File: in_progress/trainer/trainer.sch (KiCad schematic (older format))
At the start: 58 parts, among them CON1 BARREL_JACK, P1 CONN_01X04, P2 CONN_01X02, P3 CONN_01X03, P4 USB_A, P5 CONN_01X02, P6 CONN_01X03, P7 CONN_02X08, Q1 2N3904, U1 ULN2803A, U2 LM7805, U3 ULN2803A, U4 ULN2803A, X1 Buzzer_Son

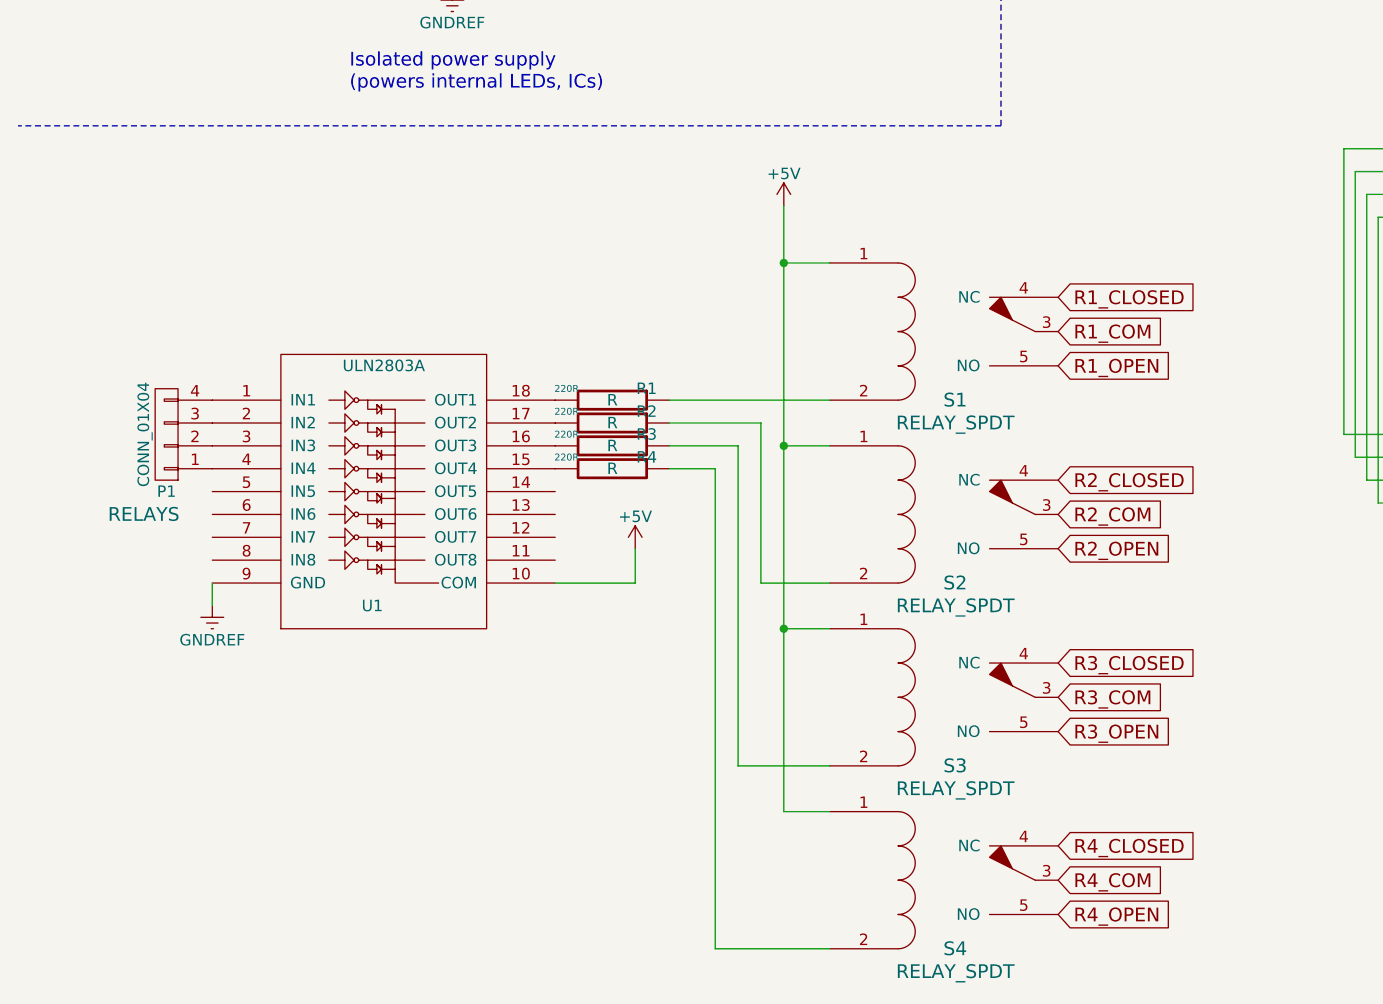
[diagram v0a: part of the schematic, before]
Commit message: .
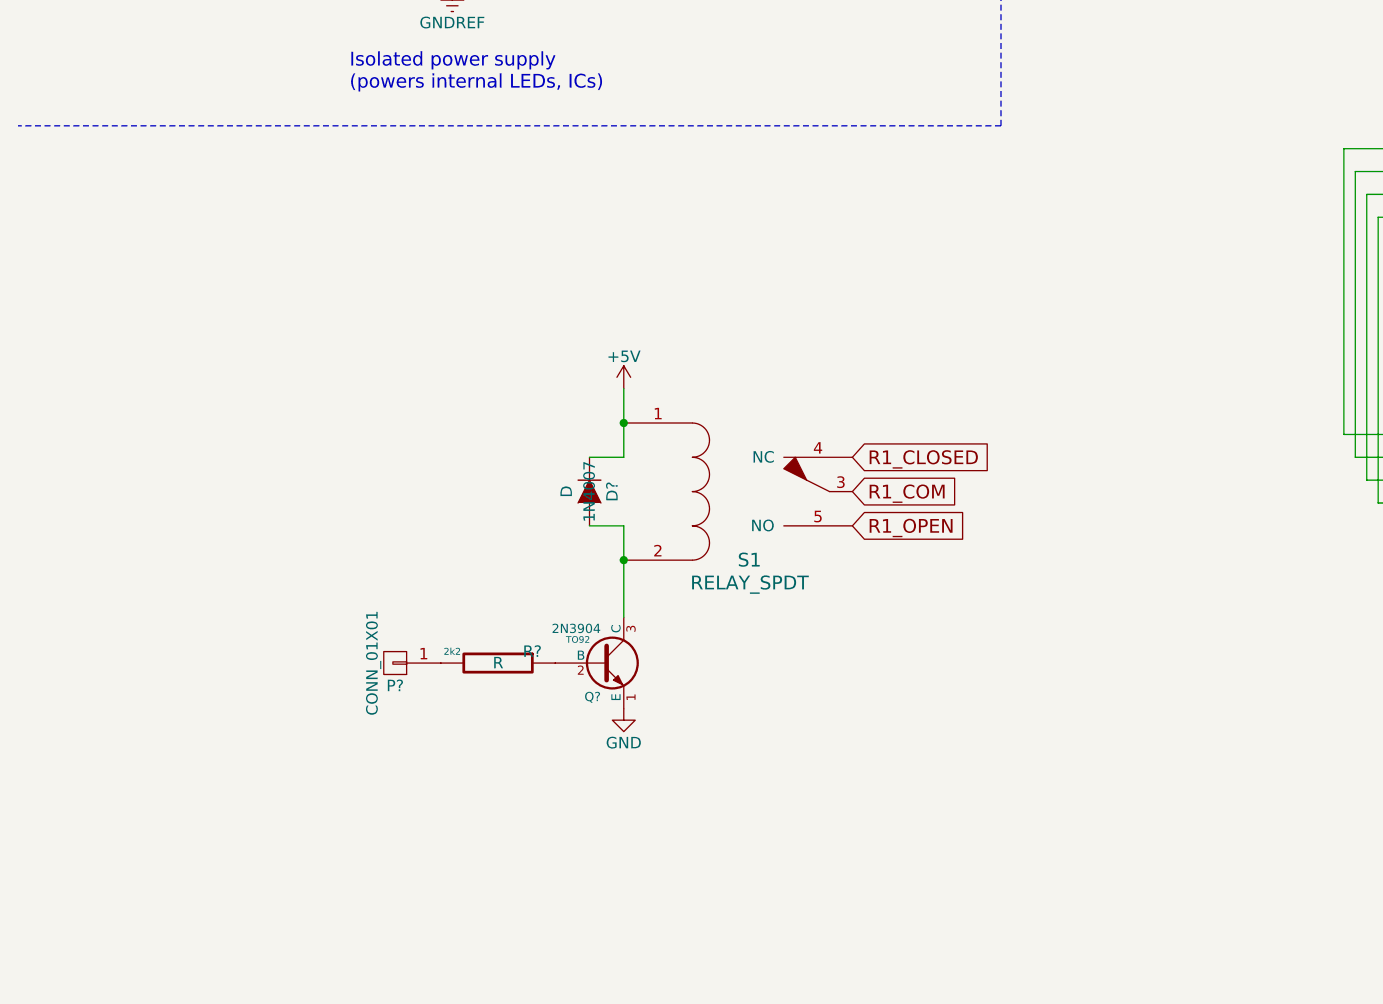
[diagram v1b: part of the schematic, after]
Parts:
- removed P1: CONN_01X04, RELAYS, symbol CONN_01X04
- removed R1, R2, R3, R4: R, 220R, symbol R-RESCUE-trainer
- removed S2, S3, S4: RELAY_SPDT, symbol RELAY_SPDT
- removed U1: ULN2803A, symbol ULN2803A
- added D?: D, 1N4007, symbol D
- added P?: CONN_01X01, symbol CONN_01X01
- added Q?: 2N3904, TO92, symbol PN2222A-RESCUE-trainer
- added R?: R, 2k2, symbol R-RESCUE-trainer
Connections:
- net labels removed: R2_CLOSED, R2_COM, R2_OPEN, R3_CLOSED, R3_COM, R3_OPEN, R4_CLOSED, R4_COM, R4_OPEN
- wire segments 123 -> 109
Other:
- moved on the sheet: S1
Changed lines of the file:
@@
 F1 "inputs.sch" 60
 $EndSheet
-$Comp
-L RELAY_SPDT S1
-U 1 1 56568F0F
-P 4700 4450
-F 0 "S1" H 4700 4150 60  0000 C CNN
-F 1 "RELAY_SPDT" H 4700 4050 60  0000 C CNN
-F 2 "" H 4700 4450 60  0000 C CNN
-F 3 "" H 4700 4450 60  0000 C CNN
-	1    4700 4450
-	1    0    0    -1
-$EndComp
-$Comp
-L CONN_01X04 P1
-U 1 1 5656959C
-P 1250 4900
-F 0 "P1" H 1250 5150 50  0000 C CNN
-F 1 "CONN_01X04" V 1350 4900 50  0000 C CNN
-F 2 "RELAYS" H 1350 5250 60  0000 C CNN
-F 3 "" H 1250 4900 60  0000 C CNN
-	1    1250 4900
-	-1   0    0    1
-$EndComp
-Text GLabel 5150 4300 2    60   Input ~ 0
+Text GLabel 4250 5000 2    60   Input ~ 0
 R1_CLOSED
-Text GLabel 5150 4450 2    60   Input ~ 0
+Text GLabel 4250 5150 2    60   Input ~ 0
 R1_COM
-Text GLabel 5150 4600 2    60   Input ~ 0
+Text GLabel 4250 5300 2    60   Input ~ 0
 R1_OPEN
-$Comp
-L RELAY_SPDT S2
-U 1 1 5656BF1B
-P 4700 5250
-F 0 "S2" H 4700 4950 60  0000 C CNN
-F 1 "RELAY_SPDT" H 4700 4850 60  0000 C CNN
-F 2 "" H 4700 5250 60  0000 C CNN
-F 3 "" H 4700 5250 60  0000 C CNN
-	1    4700 5250
-	1    0    0    -1
-$EndComp
-Text GLabel 5150 5100 2    60   Input ~ 0
-R2_CLOSED
-Text GLabel 5150 5250 2    60   Input ~ 0
-R2_COM
-Text GLabel 5150 5400 2    60   Input ~ 0
-R2_OPEN
-$Comp
-L RELAY_SPDT S3
-U 1 1 5656C278
-P 4700 6050
-F 0 "S3" H 4700 5750 60  0000 C CNN
-F 1 "RELAY_SPDT" H 4700 5650 60  0000 C CNN
-F 2 "" H 4700 6050 60  0000 C CNN
-F 3 "" H 4700 6050 60  0000 C CNN
-	1    4700 6050
-	1    0    0    -1
-$EndComp
-Text GLabel 5150 5900 2    60   Input ~ 0
-R3_CLOSED
-Text GLabel 5150 6050 2    60   Input ~ 0
-R3_COM
-Text GLabel 5150 6200 2    60   Input ~ 0
-R3_OPEN
-$Comp
-L RELAY_SPDT S4
-U 1 1 5656C28D
-P 4700 6850
-F 0 "S4" H 4700 6550 60  0000 C CNN
-F 1 "RELAY_SPDT" H 4700 6450 60  0000 C CNN
-F 2 "" H 4700 6850 60  0000 C CNN
-F 3 "" H 4700 6850 60  0000 C CNN
-	1    4700 6850
-	1    0    0    -1
-$EndComp
-Text GLabel 5150 6700 2    60   Input ~ 0
-R4_CLOSED
-Text GLabel 5150 6850 2    60   Input ~ 0
-R4_COM
-Text GLabel 5150 7000 2    60   Input ~ 0
-R4_OPEN
 $Comp
 L LM7805 U2
@@
 $EndComp
 $Comp
-L R-RESCUE-trainer R1
-U 1 1 5659DCCE
-P 3200 4750
-F 0 "R1" V 3150 4900 50  0000 C CNN
-F 1 "R" V 3200 4750 50  0000 C CNN
-F 2 "220R" V 3150 4550 30  0000 C CNN
-F 3 "" H 3200 4750 30  0000 C CNN
-	1    3200 4750
-	0    1    1    0
-$EndComp
-$Comp
-L R-RESCUE-trainer R2
-U 1 1 5659E1A6
-P 3200 4850
-F 0 "R2" V 3150 5000 50  0000 C CNN
-F 1 "R" V 3200 4850 50  0000 C CNN
-F 2 "220R" V 3150 4650 30  0000 C CNN
-F 3 "" H 3200 4850 30  0000 C CNN
-	1    3200 4850
-	0    1    1    0
-$EndComp
-$Comp
-L R-RESCUE-trainer R3
-U 1 1 5659E1E3
-P 3200 4950
-F 0 "R3" V 3150 5100 50  0000 C CNN
-F 1 "R" V 3200 4950 50  0000 C CNN
-F 2 "220R" V 3150 4750 30  0000 C CNN
-F 3 "" H 3200 4950 30  0000 C CNN
-	1    3200 4950
-	0    1    1    0
-$EndComp
-$Comp
-L R-RESCUE-trainer R4
-U 1 1 5659E227
-P 3200 5050
-F 0 "R4" V 3150 5200 50  0000 C CNN
-F 1 "R" V 3200 5050 50  0000 C CNN
-F 2 "220R" V 3150 4850 30  0000 C CNN
-F 3 "" H 3200 5050 30  0000 C CNN
-	1    3200 5050
-	0    1    1    0
-$EndComp
-$Comp
-L ULN2803A U1
-U 1 1 5659B908
-P 2200 5150
-F 0 "U1" H 2150 4650 50  0000 C CNN
-F 1 "ULN2803A" H 2200 5700 50  0000 C CNN
-F 2 "" H 2200 5150 60  0000 C CNN
-F 3 "" H 2200 5150 60  0000 C CNN
-	1    2200 5150
-	1    0    0    -1
-$EndComp
-$Comp
 L +5V #PWR8
 U 1 1 565A0518
-P 3950 3900
-F 0 "#PWR8" H 3950 3750 50  0001 C CNN
-F 1 "+5V" H 3950 4040 50  0000 C CNN
-F 2 "" H 3950 3900 60  0000 C CNN
-F 3 "" H 3950 3900 60  0000 C CNN
-	1    3950 3900
-	1    0    0    -1
-$EndComp
-$Comp
-L GNDREF #PWR3
-U 1 1 565A1ACC
-P 1450 5650
-F 0 "#PWR3" H 1450 5400 50  0001 C CNN
-F 1 "GNDREF" H 1450 5500 50  0000 C CNN
-F 2 "" H 1450 5650 60  0000 C CNN
-F 3 "" H 1450 5650 60  0000 C CNN
-	1    1450 5650
-	1    0    0    -1
-$EndComp
-$Comp
-L +5V #PWR6
-U 1 1 565A1B8D
-P 3300 5400
-F 0 "#PWR6" H 3300 5250 50  0001 C CNN
-F 1 "+5V" H 3300 5540 50  0000 C CNN
-F 2 "" H 3300 5400 60  0000 C CNN
-F 3 "" H 3300 5400 60  0000 C CNN
-	1    3300 5400
+P 3250 4700
+F 0 "#PWR8" H 3250 4550 50  0001 C CNN
+F 1 "+5V" H 3250 4840 50  0000 C CNN
+F 2 "" H 3250 4700 60  0000 C CNN
+F 3 "" H 3250 4700 60  0000 C CNN
+	1    3250 4700
 	1    0    0    -1
 $EndComp
@@
 	3500 2850 3500 2500
 Wire Wire Line
-	3950 3900 3950 6550
-Wire Wire Line
-	3950 4150 4150 4150
-Wire Wire Line
-	3950 4950 4150 4950
-Connection ~ 3950 4150
-Wire Wire Line
-	3950 5750 4150 5750
-Connection ~ 3950 4950
-Wire Wire Line
-	3950 6550 4150 6550
-Connection ~ 3950 5750
-Wire Wire Line
-	4150 4750 3450 4750
-Wire Wire Line
-	4150 5550 3850 5550
-Wire Wire Line
-	3850 5550 3850 4850
-Wire Wire Line
-	3850 4850 3450 4850
-Wire Wire Line
-	4150 6350 3750 6350
-Wire Wire Line
-	3750 6350 3750 4950
-Wire Wire Line
-	3750 4950 3450 4950
-Wire Wire Line
-	4150 7150 3650 7150
-Wire Wire Line
-	3650 7150 3650 5050
-Wire Wire Line
-	3650 5050 3450 5050
-Wire Wire Line
-	1450 5650 1450 5550
-Wire Wire Line
-	2950 5550 3300 5550
-Wire Wire Line
-	3300 5550 3300 5400
-Wire Wire Line
 	1350 1000 1350 1200
 Wire Wire Line
@@
 Wire Notes Line
 	4900 3550 4900 600
+$Comp
+L PN2222A-RESCUE-trainer Q?
+U 1 1 568E687A
+P 3150 5900
+F 0 "Q?" H 3150 5752 40  0000 R CNN
+F 1 "2N3904" H 3150 6050 40  0000 R CNN
+F 2 "TO92" H 3050 6002 29  0000 C CNN
+F 3 "~" H 3150 5900 60  0000 C CNN
+	1    3150 5900
+	1    0    0    -1
+$EndComp
+$Comp
+L R-RESCUE-trainer R?
+U 1 1 568E6880
+P 2700 5900
+F 0 "R?" V 2650 6050 50  0000 C CNN
+F 1 "R" V 2700 5900 50  0000 C CNN
+F 2 "2k2" V 2650 5700 30  0000 C CNN
+F 3 "" H 2700 5900 30  0000 C CNN
+	1    2700 5900
+	0    1    1    0
+$EndComp
+$Comp
+L GND #PWR?
+U 1 1 568E6886
+P 3250 6100
+F 0 "#PWR?" H 3250 5850 50  0001 C CNN
+F 1 "GND" H 3250 5950 50  0000 C CNN
+F 2 "" H 3250 6100 50  0000 C CNN
+F 3 "" H 3250 6100 50  0000 C CNN
+	1    3250 6100
+	1    0    0    -1
+$EndComp
+$Comp
+L D D?
+U 1 1 568E6A1E
+P 3100 5150
+F 0 "D?" H 3100 5250 50  0000 C CNN
+F 1 "D" H 3100 5050 50  0000 C CNN
+F 2 "1N4007" H 3100 5150 50  0000 C CNN
+F 3 "" H 3100 5150 50  0000 C CNN
+	1    3100 5150
+	0    1    1    0
+$EndComp
+$Comp
+L RELAY_SPDT S1
+U 1 1 56568F0F
+P 3800 5150
+F 0 "S1" H 3800 4850 60  0000 C CNN
+F 1 "RELAY_SPDT" H 3800 4750 60  0000 C CNN
+F 2 "" H 3800 5150 60  0000 C CNN
+F 3 "" H 3800 5150 60  0000 C CNN
+	1    3800 5150
+	1    0    0    -1
+$EndComp
+Wire Wire Line
+	3250 5300 3250 5700
+Wire Wire Line
+	3250 4700 3250 5000
+Wire Wire Line
+	3250 5300 3100 5300
+Connection ~ 3250 5450
+Wire Wire Line
+	3250 5000 3100 5000
+Connection ~ 3250 4850
+$Comp
+L CONN_01X01 P?
+U 1 1 568E752E
+P 2250 5900
+F 0 "P?" H 2250 6000 50  0000 C CNN
+F 1 "CONN_01X01" V 2350 5900 50  0000 C CNN
+F 2 "" H 2250 5900 50  0000 C CNN
+F 3 "" H 2250 5900 50  0000 C CNN
+	1    2250 5900
+	-1   0    0    1
+$EndComp
 $EndSCHEMATC

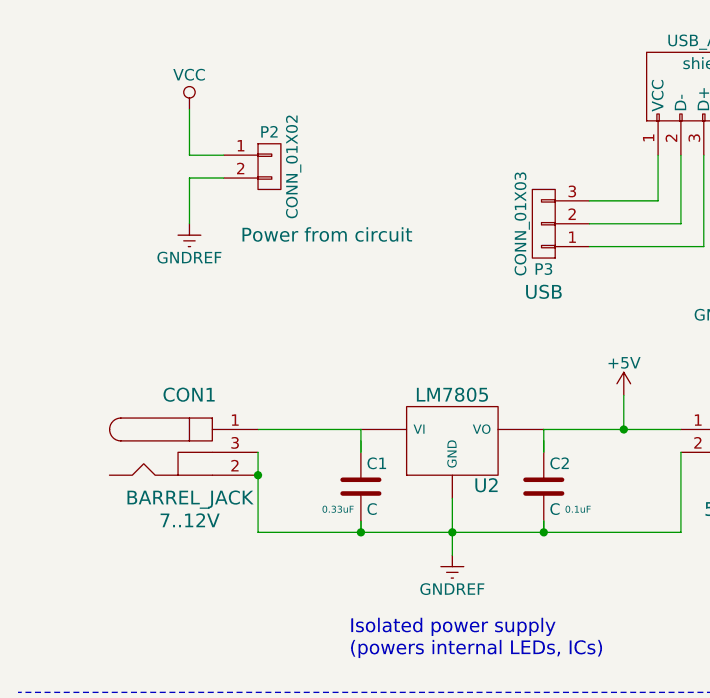
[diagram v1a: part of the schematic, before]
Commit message: .
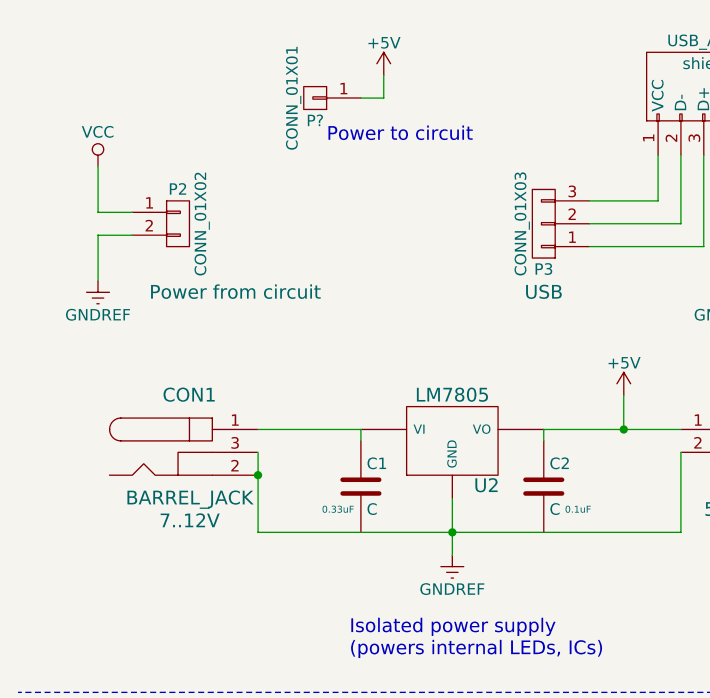
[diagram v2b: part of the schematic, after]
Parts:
- added P?: CONN_01X01, symbol CONN_01X01
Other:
- note added: "Power to circuit"
- moved on the sheet: P2
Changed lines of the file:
@@
 L CONN_01X02 P2
 U 1 1 565A8A8C
-P 1700 1250
-F 0 "P2" H 1700 1400 50  0000 C CNN
-F 1 "CONN_01X02" V 1800 1250 50  0000 C CNN
-F 2 "Power from circuit" H 1950 950 60  0000 C CNN
-F 3 "" H 1700 1250 60  0000 C CNN
-	1    1700 1250
+P 1300 1500
+F 0 "P2" H 1300 1650 50  0000 C CNN
+F 1 "CONN_01X02" V 1400 1500 50  0000 C CNN
+F 2 "Power from circuit" H 1550 1200 60  0000 C CNN
+F 3 "" H 1300 1500 60  0000 C CNN
+	1    1300 1500
 	1    0    0    -1
 $EndComp
@@
 L VCC #PWR1
 U 1 1 565A8B1D
-P 1350 1000
-F 0 "#PWR1" H 1350 850 50  0001 C CNN
-F 1 "VCC" H 1350 1150 50  0000 C CNN
-F 2 "" H 1350 1000 60  0000 C CNN
-F 3 "" H 1350 1000 60  0000 C CNN
-	1    1350 1000
+P 950 1250
+F 0 "#PWR1" H 950 1100 50  0001 C CNN
+F 1 "VCC" H 950 1400 50  0000 C CNN
+F 2 "" H 950 1250 60  0000 C CNN
+F 3 "" H 950 1250 60  0000 C CNN
+	1    950  1250
 	1    0    0    -1
 $EndComp
@@
 L GNDREF #PWR2
 U 1 1 565A8FBD
-P 1350 1500
-F 0 "#PWR2" H 1350 1250 50  0001 C CNN
-F 1 "GNDREF" H 1350 1350 50  0000 C CNN
-F 2 "" H 1350 1500 60  0000 C CNN
-F 3 "" H 1350 1500 60  0000 C CNN
-	1    1350 1500
+P 950 1750
+F 0 "#PWR2" H 950 1500 50  0001 C CNN
+F 1 "GNDREF" H 950 1600 50  0000 C CNN
+F 2 "" H 950 1750 60  0000 C CNN
+F 3 "" H 950 1750 60  0000 C CNN
+	1    950  1750
 	1    0    0    -1
 $EndComp
@@
 	1650 2400 2100 2400
 Wire Wire Line
-	2900 2500 2900 2400
-Wire Wire Line
 	2900 2400 3500 2400
-Wire Wire Line
-	2100 2400 2100 2500
 Wire Wire Line
 	3250 2400 3250 2250
@@
 	1650 2850 3500 2850
 Wire Wire Line
-	2900 2850 2900 2800
-Wire Wire Line
 	2500 2700 2500 2950
-Connection ~ 2900 2850
 Connection ~ 2500 2850
-Wire Wire Line
-	2100 2850 2100 2800
-Connection ~ 2100 2850
 Wire Wire Line
 	3500 1500 3100 1500
@@
 	3500 2850 3500 2500
 Wire Wire Line
-	1350 1000 1350 1200
-Wire Wire Line
-	1350 1200 1500 1200
-Wire Wire Line
-	1350 1500 1350 1300
-Wire Wire Line
-	1350 1300 1500 1300
+	950  1250 950  1450
+Wire Wire Line
+	950  1450 1100 1450
+Wire Wire Line
+	950  1750 950  1550
+Wire Wire Line
+	950  1550 1100 1550
 Wire Wire Line
 	5950 1850 6050 1850
@@
 	-1   0    0    1
 $EndComp
+Wire Wire Line
+	2100 2400 2100 2450
+Wire Wire Line
+	2900 2450 2900 2400
+$Comp
+L CONN_01X01 P?
+U 1 1 566E190D
+P 1900 950
+F 0 "P?" H 1900 1050 50  0000 C CNN
+F 1 "CONN_01X01" V 2000 950 50  0000 C CNN
+F 2 "" H 1900 950 50  0000 C CNN
+F 3 "" H 1900 950 50  0000 C CNN
+	1    1900 950
+	-1   0    0    1
+$EndComp
+$Comp
+L +5V #PWR?
+U 1 1 566E2984
+P 2200 850
+F 0 "#PWR?" H 2200 700 50  0001 C CNN
+F 1 "+5V" H 2200 990 50  0000 C CNN
+F 2 "" H 2200 850 50  0000 C CNN
+F 3 "" H 2200 850 50  0000 C CNN
+	1    2200 850
+	1    0    0    -1
+$EndComp
+Wire Wire Line
+	2100 950  2200 950
+Wire Wire Line
+	2200 950  2200 850
+Text Notes 1950 1150 0    60   ~ 0
+Power to circuit
 $EndSCHEMATC
